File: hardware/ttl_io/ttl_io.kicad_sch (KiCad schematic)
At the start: 32 parts, among them J13 Conn_02x08_Counter_Clockwise, J14 Conn_02x08_Counter_Clockwise, SW2 SW_SPDT, SW3 SW_SPDT, U14 74CBTLV3245, U16 74CBTLV3245, U17 74CBTLV3245, U18 74LVC1G04, U19 TXB0108DQSR

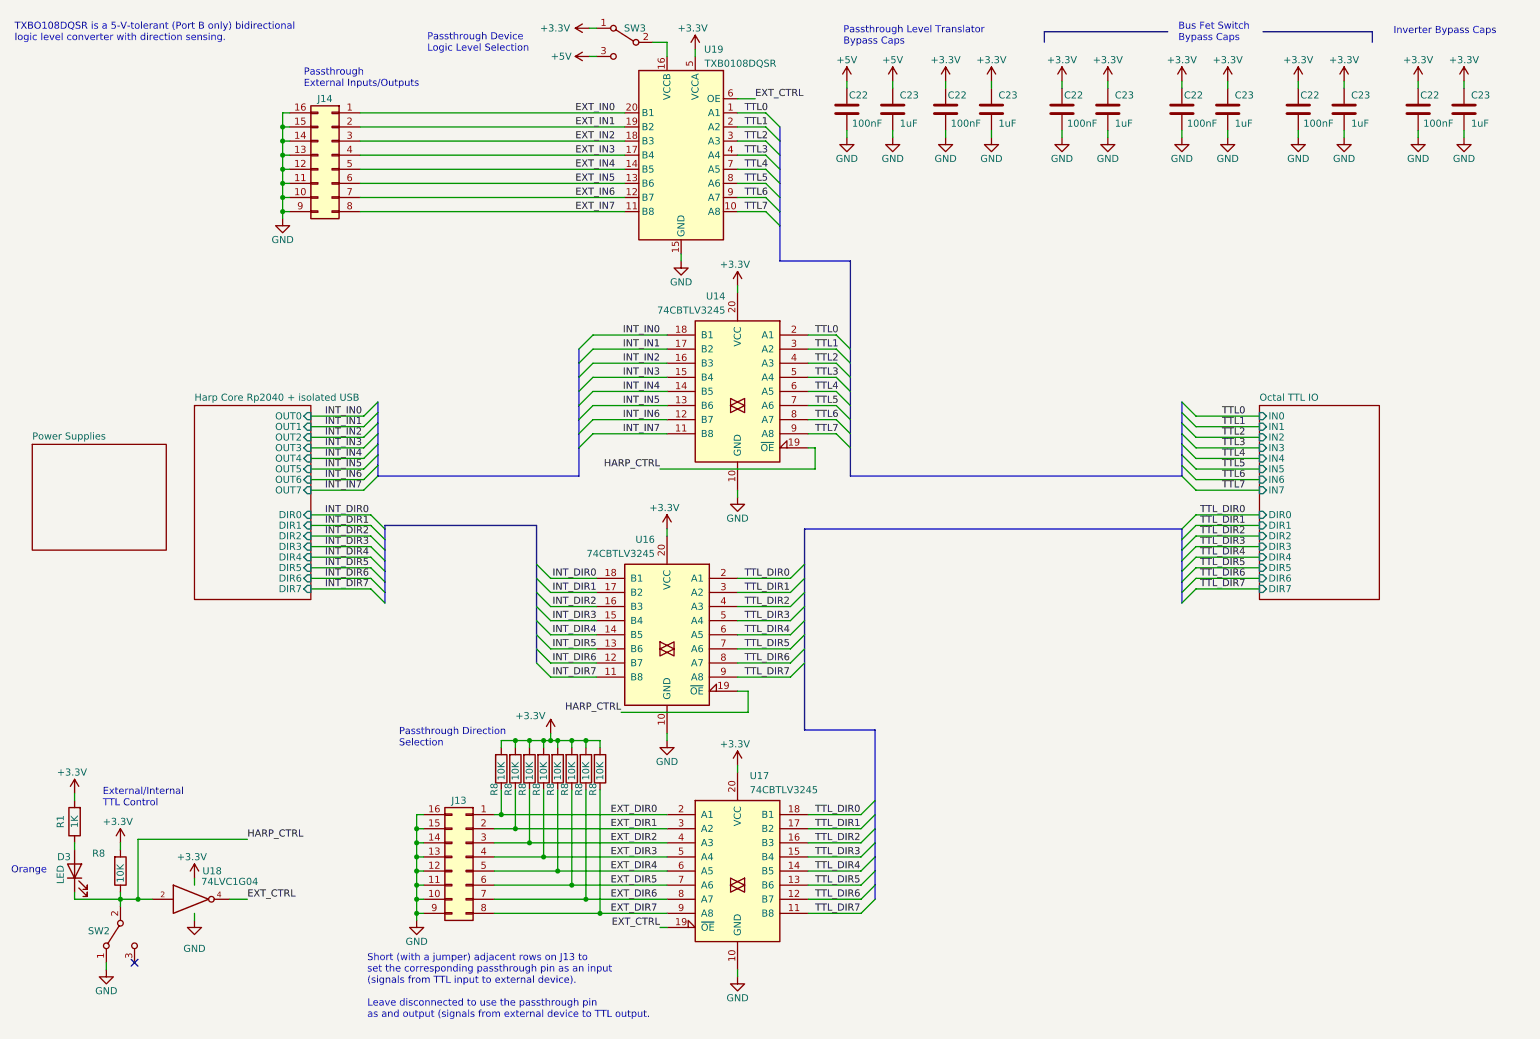
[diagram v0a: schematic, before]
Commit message: update layout
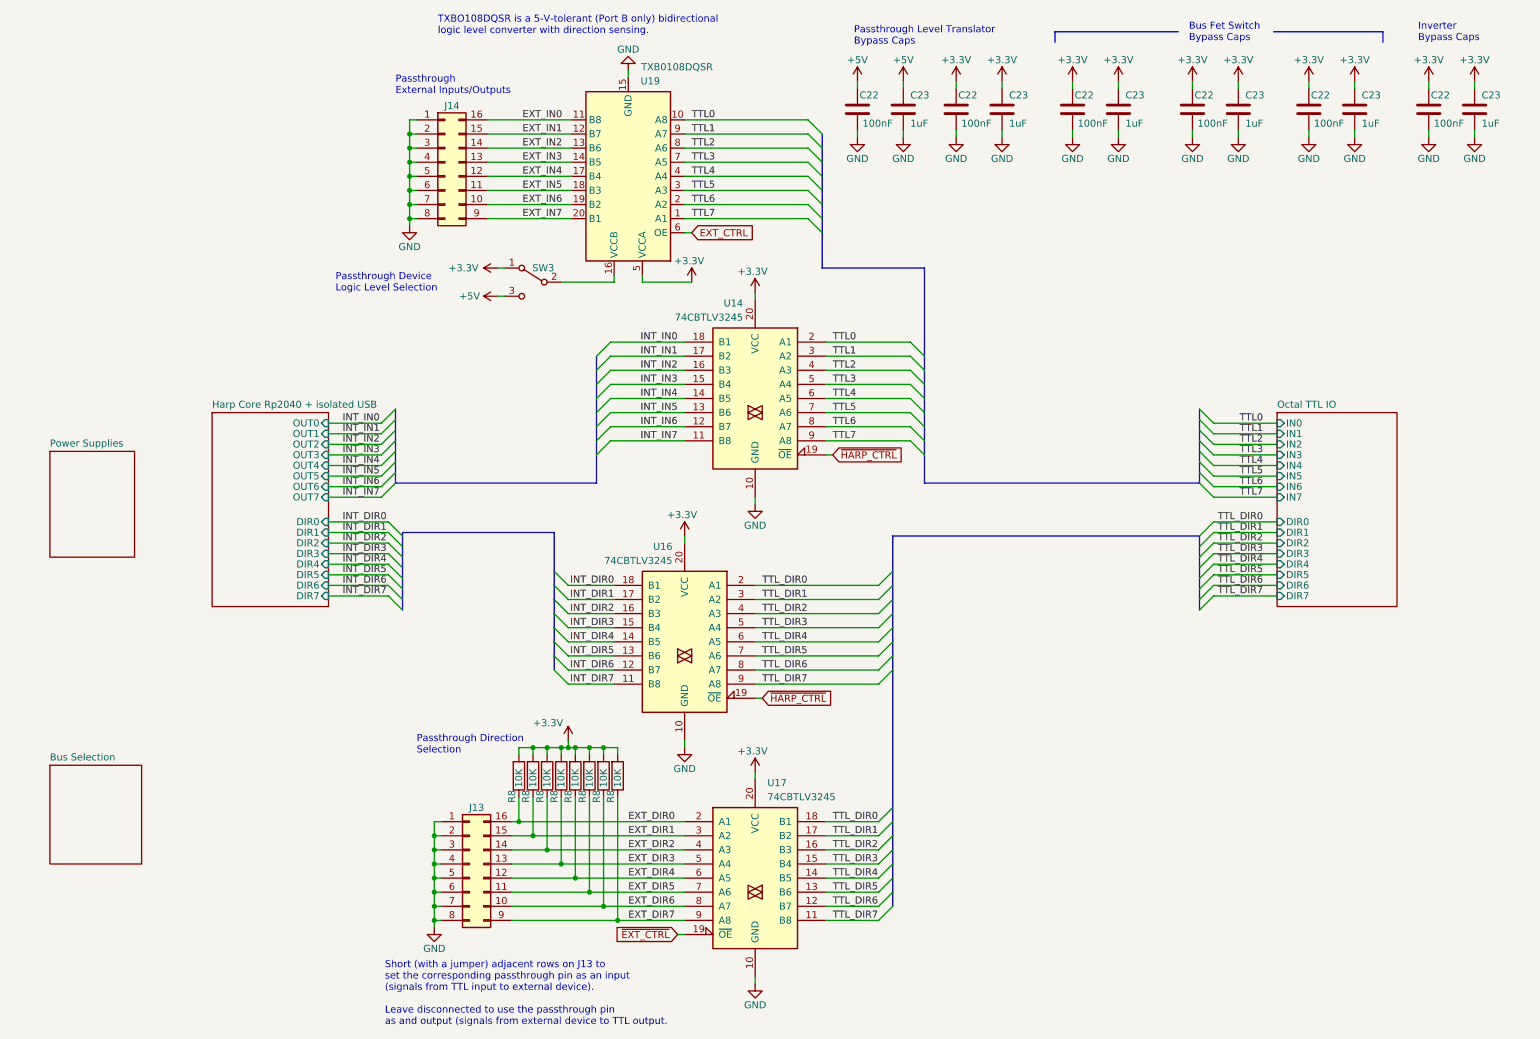
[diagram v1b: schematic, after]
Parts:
- removed D3: LED, LED_SMD:LED_0603_1608Metric, symbol Device:LED
- removed R1: 1K, Resistor_SMD:R_0402_1005Metric, symbol Device:R
- removed R8: 10K, Resistor_SMD:R_0402_1005Metric, symbol Device:R
- removed SW2: SW_SPDT, Button_Switch_SMD:SW_SPDT_CK-JS102011SAQN, symbol Switch:SW_SPDT
- removed U18: 74LVC1G04, Package_TO_SOT_SMD:SOT-23-5, symbol 74xGxx:74LVC1G04
- J13, J14: footprint Connector_PinHeader_2.54mm:PinHeader_2x08_P2.54mm_Vertical_SMD -> kicad_component_library:PinHeader_2x08_P2.54mm_Horizontal_SMD
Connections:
- net EXT_CTRL: no longer U17.19 (~{OE})
- net EXT_DIR0: now also J13.16 (Pin_16); no longer J13.1 (Pin_1)
- net EXT_DIR1: now also J13.15 (Pin_15); no longer J13.2 (Pin_2)
- net EXT_DIR2: now also J13.14 (Pin_14); no longer J13.3 (Pin_3)
- net EXT_DIR3: now also J13.13 (Pin_13); no longer J13.4 (Pin_4)
- net EXT_DIR4: now also J13.12 (Pin_12); no longer J13.5 (Pin_5)
- net EXT_DIR5: now also J13.11 (Pin_11); no longer J13.6 (Pin_6)
- net EXT_DIR6: now also J13.10 (Pin_10); no longer J13.7 (Pin_7)
- net EXT_DIR7: now also J13.9 (Pin_9); no longer J13.8 (Pin_8)
- net EXT_IN0: now also J14.16 (Pin_16), U19.11 (B8); no longer J14.1 (Pin_1), U19.20 (B1)
- net EXT_IN1: now also J14.15 (Pin_15), U19.12 (B7); no longer J14.2 (Pin_2), U19.19 (B2)
- net EXT_IN2: now also J14.14 (Pin_14), U19.13 (B6); no longer J14.3 (Pin_3), U19.18 (B3)
- net EXT_IN3: now also J14.13 (Pin_13), U19.14 (B5); no longer J14.4 (Pin_4), U19.17 (B4)
- net EXT_IN4: now also J14.12 (Pin_12), U19.17 (B4); no longer J14.5 (Pin_5), U19.14 (B5)
- net EXT_IN5: now also J14.11 (Pin_11), U19.18 (B3); no longer J14.6 (Pin_6), U19.13 (B6)
- net EXT_IN6: now also J14.10 (Pin_10), U19.19 (B2); no longer J14.7 (Pin_7), U19.12 (B7)
- net EXT_IN7: now also J14.9 (Pin_9), U19.20 (B1); no longer J14.8 (Pin_8), U19.11 (B8)
- net GND: now also J13.1 (Pin_1), J13.2 (Pin_2), J13.3 (Pin_3), J13.4 (Pin_4), J13.5 (Pin_5), J13.6 (Pin_6), J13.7 (Pin_7), J13.8 (Pin_8), J14.1 (Pin_1), J14.2 (Pin_2), J14.3 (Pin_3), J14.4 (Pin_4), J14.5 (Pin_5), J14.6 (Pin_6), J14.7 (Pin_7), J14.8 (Pin_8); no longer J13.10 (Pin_10), J13.11 (Pin_11), J13.12 (Pin_12), J13.13 (Pin_13), J13.14 (Pin_14), J13.15 (Pin_15), J13.16 (Pin_16), J13.9 (Pin_9), J14.10 (Pin_10), J14.11 (Pin_11), J14.12 (Pin_12), J14.13 (Pin_13), J14.14 (Pin_14), J14.15 (Pin_15), J14.16 (Pin_16), J14.9 (Pin_9)
- net TTL0: now also U19.10 (A8); no longer U19.1 (A1)
- net TTL1: now also U19.9 (A7); no longer U19.2 (A2)
- net TTL2: now also U19.8 (A6); no longer U19.3 (A3)
- net TTL3: now also U19.7 (A5); no longer U19.4 (A4)
- net TTL4: now also U19.4 (A4); no longer U19.7 (A5)
- net TTL5: now also U19.3 (A3); no longer U19.8 (A6)
- net TTL6: now also U19.2 (A2); no longer U19.9 (A7)
- net TTL7: now also U19.1 (A1); no longer U19.10 (A8)
- net HARP_CTRL renamed ~{HARP_CTRL}
- new net ~{EXT_CTRL}: U17.19 (~{OE})
- no-connect marks 1 -> 0
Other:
- added sheet Bus Selection (bus_selection.kicad_sch)
- note removed: "External/Internal TTL Control"
- note removed: "Orange"
- moved on the sheet: C22, C23, J13, J14, R8, SW3, U14, U16, U17, U19
